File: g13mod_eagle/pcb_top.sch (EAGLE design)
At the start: 20 parts

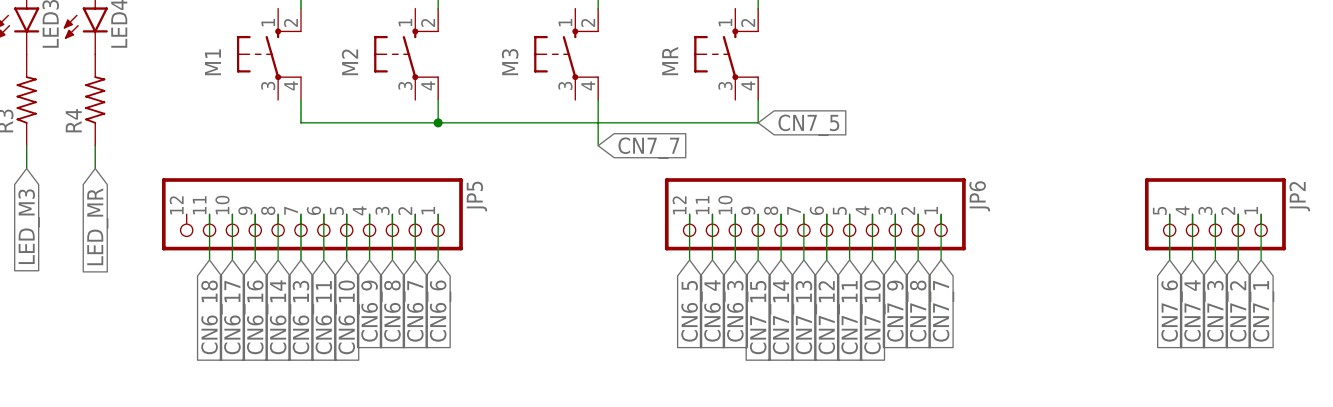
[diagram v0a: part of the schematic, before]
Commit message: Edit connector
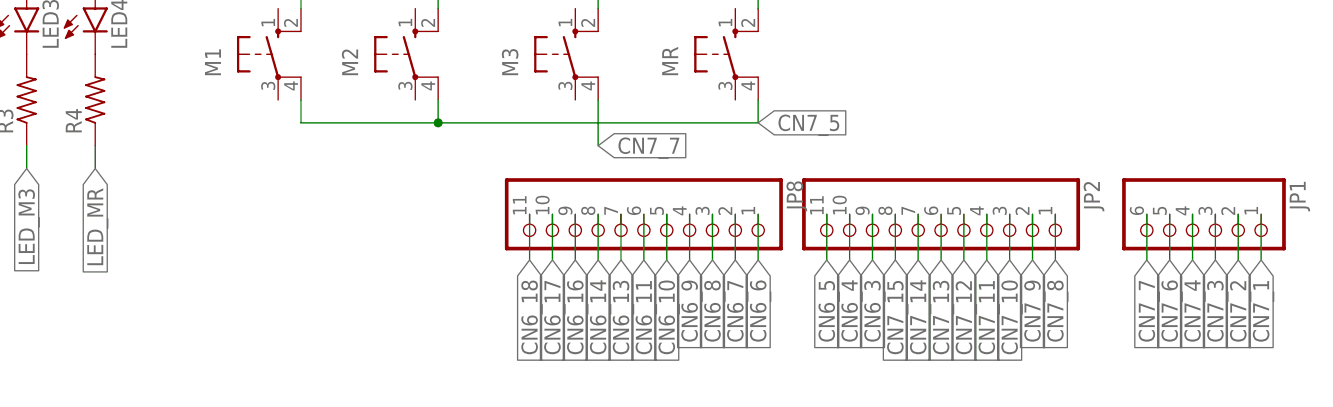
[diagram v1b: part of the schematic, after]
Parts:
- removed JP5, JP6: (no value), pinhead-half-pitch:THROUHOLE12
- added JP1: (no value), pinhead-half-pitch:THROUHOLE06
- added JP8: (no value), pinhead-half-pitch:THROUHOLE11
- JP2: device pinhead-half-pitch:THROUHOLE05 -> pinhead-half-pitch:THROUHOLE11
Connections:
- net CN6_10: now also JP8.5; no longer JP5.5
- net CN6_11: now also JP8.6; no longer JP5.6
- net CN6_13: now also JP8.7; no longer JP5.7
- net CN6_14: now also JP8.8; no longer JP5.8
- net CN6_16: now also JP8.9; no longer JP5.9
- net CN6_17: now also JP8.10; no longer JP5.10
- net CN6_18: now also JP8.11; no longer JP5.11
- net CN6_3: now also JP2.9; no longer JP6.10
- net CN6_4: now also JP2.10; no longer JP6.11
- net CN6_5: now also JP2.11; no longer JP6.12
- net CN6_6: now also JP8.1; no longer JP5.1
- net CN6_7: now also JP8.2; no longer JP5.2
- net CN6_8: now also JP8.3; no longer JP5.3
- net CN6_9: now also JP8.4; no longer JP5.4
- net CN7_1: now also JP1.1; no longer JP2.1
- net CN7_10: now also JP2.3; no longer JP6.4
- net CN7_11: now also JP2.4; no longer JP6.5
- net CN7_12: now also JP2.5; no longer JP6.6
- net CN7_13: now also JP2.6; no longer JP6.7
- net CN7_14: now also JP2.7; no longer JP6.8
- net CN7_15: now also JP2.8; no longer JP6.9
- net CN7_2: now also JP1.2; no longer JP2.2
- net CN7_3: now also JP1.3; no longer JP2.3
- net CN7_4: now also JP1.4; no longer JP2.4
- net CN7_6: now also JP1.5; no longer JP2.5
- net CN7_7: now also JP1.6; no longer JP6.1
- net CN7_8: now also JP2.1; no longer JP6.2
- net CN7_9: now also JP2.2; no longer JP6.3
